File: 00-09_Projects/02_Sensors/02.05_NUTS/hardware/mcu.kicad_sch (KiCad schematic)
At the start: 28 parts, among them J3 Conn_01x06_Pin, J4 SHF-107-01-L-D-SM, SW1 450404015514, SW2 TL3301EF160QG, U3 STM32F302C8Tx, U4 74HC2G32DP, Y1 RH100-16.000-9-1010-TR

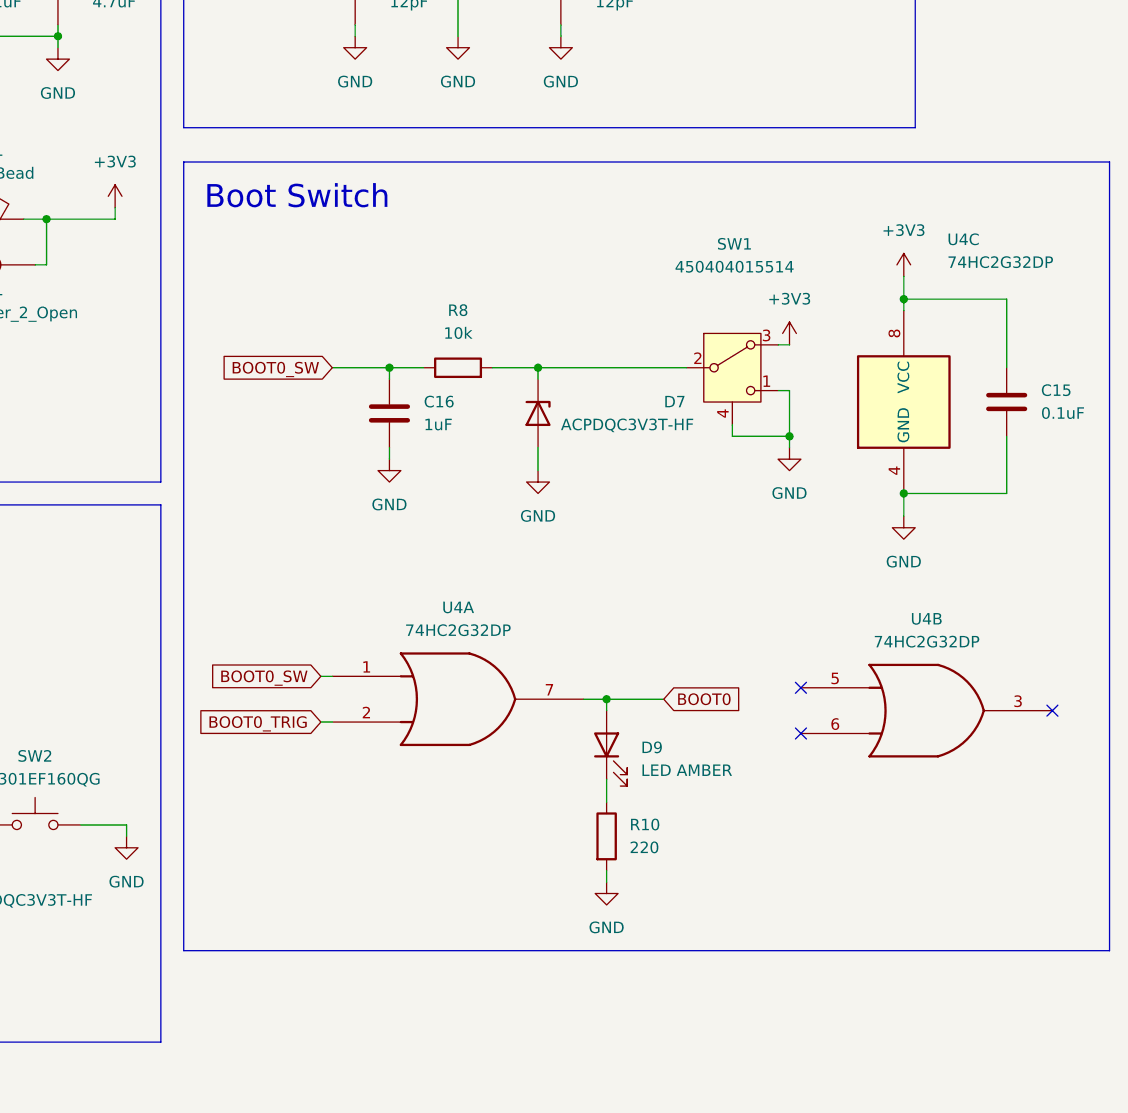
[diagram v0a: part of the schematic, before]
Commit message: extra changes
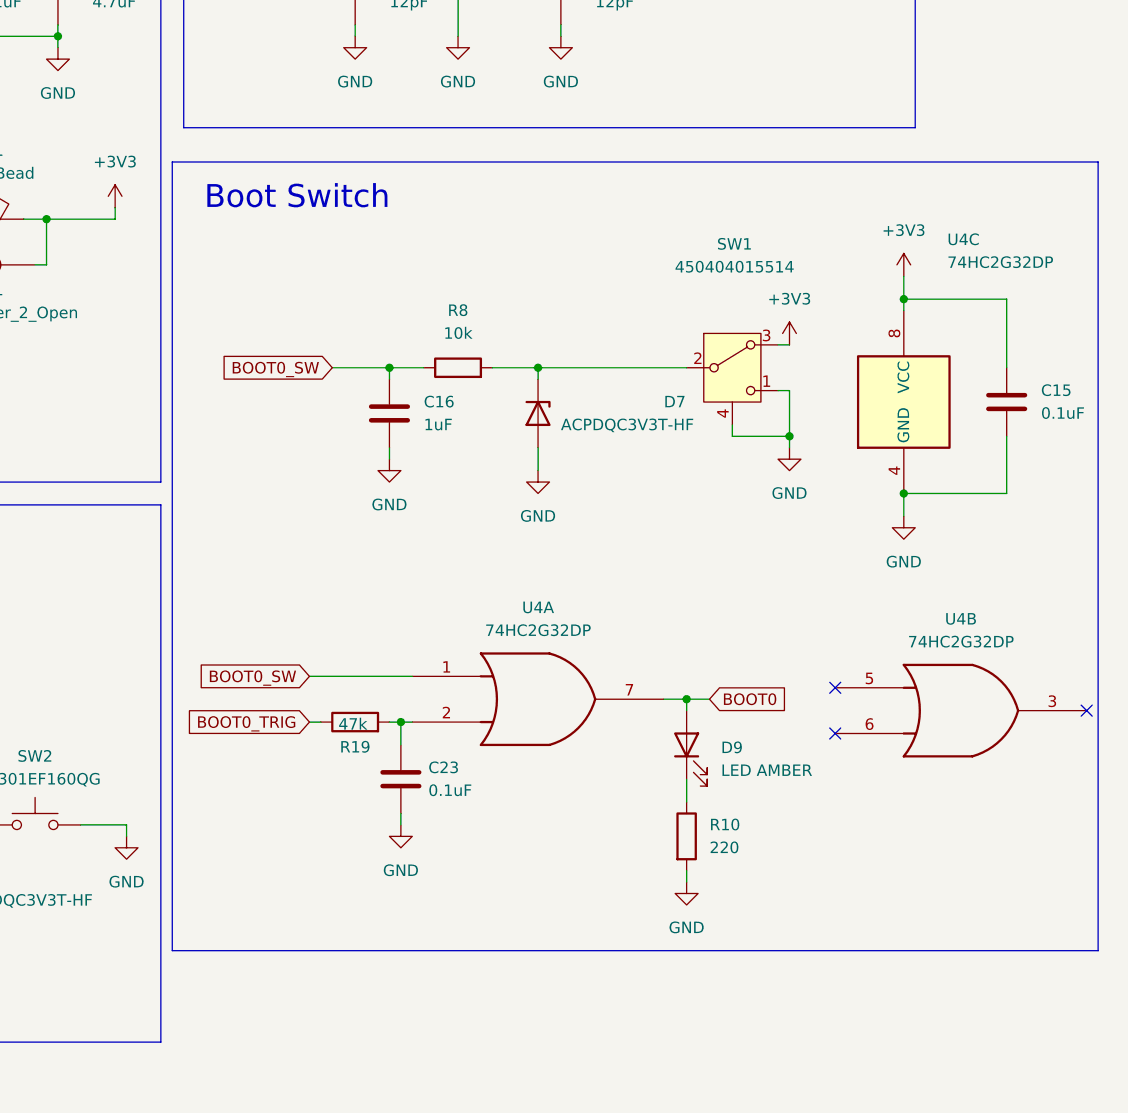
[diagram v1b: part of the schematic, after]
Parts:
- added C23: 0.1uF, Capacitor_SMD:C_0603_1608Metric_Pad1.08x0.95mm_HandSolder, symbol Device:C
- added R19: 47k, Resistor_SMD:R_0402_1005Metric_Pad0.72x0.64mm_HandSolder, symbol Device:R
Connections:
- net BOOT0_TRIG: now also R19.1; no longer U4.2
- net GND: now also C23.2
- new net: C23.1, R19.2, U4.2
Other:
- moved on the sheet: D9, R10, U4A, U4B
